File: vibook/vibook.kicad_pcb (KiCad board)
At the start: 2 copper layers, 15 x 89.5 mm, 53 parts, among them IC3 STLQ020C33R, J1 Conn_ARM_JTAG_SWD_10, SW3 SW_Push, U2 STM32L011K4Ux, U3 MPR121QR2, U5 MPR121QR2

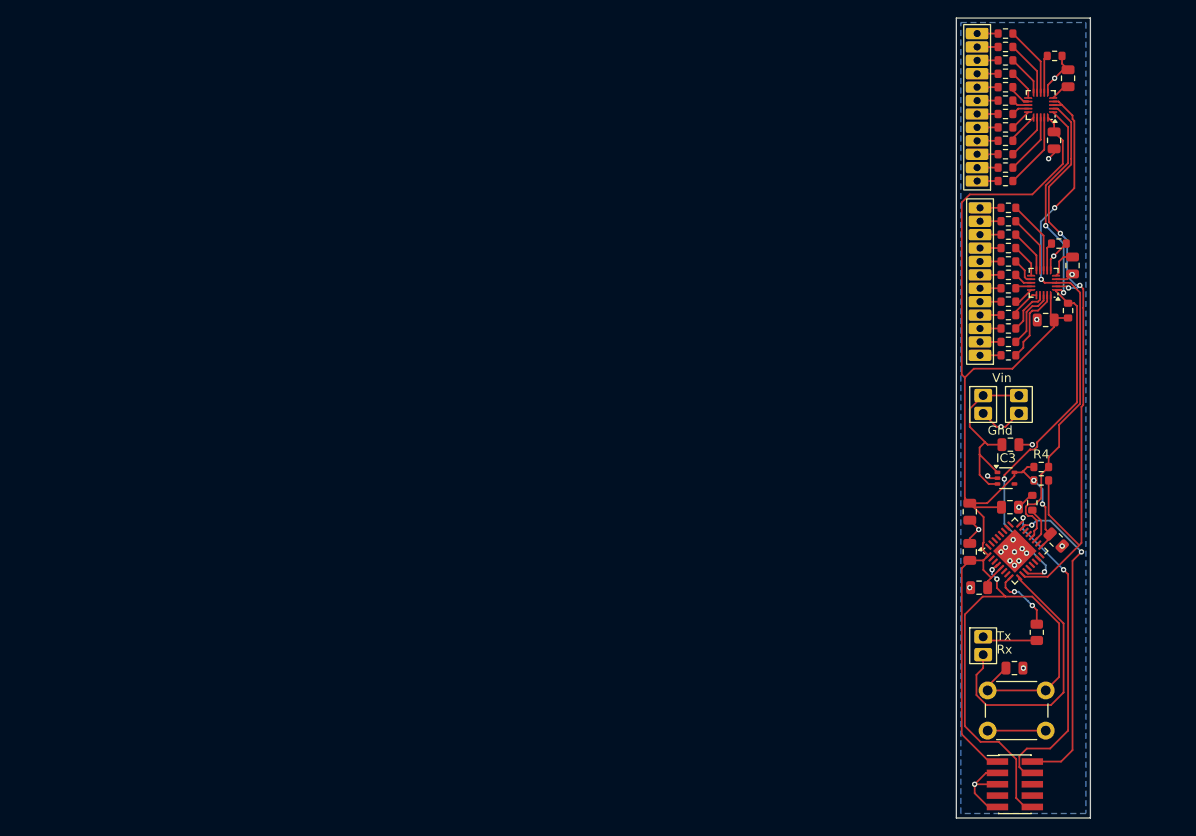
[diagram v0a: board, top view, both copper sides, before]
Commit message: updated board design
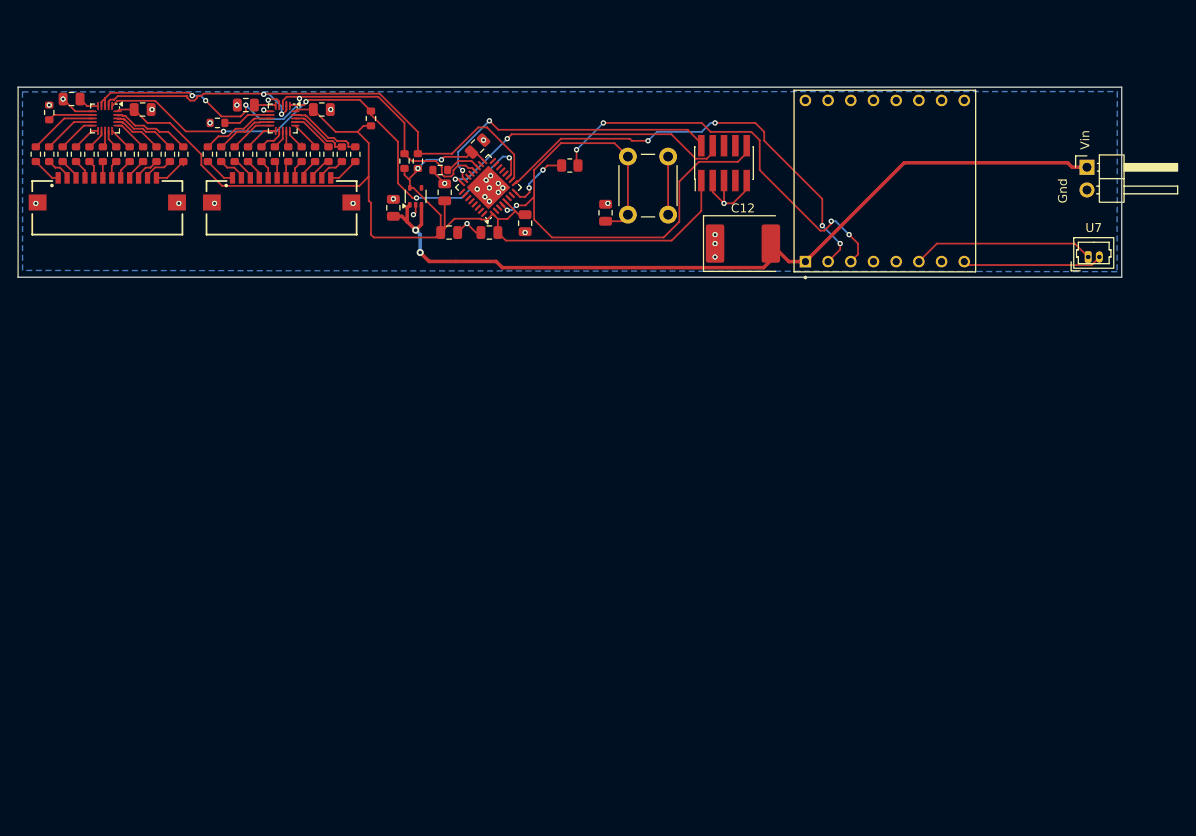
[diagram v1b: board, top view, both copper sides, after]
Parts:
- removed U1, U4: ~, jlc:12matrix
- added C12: 470u, Capacitor_Tantalum_SMD:CP_EIA-7360-38_Kemet-E, F.Cu at (102.6, 111.5)
- added J2: 6861XX148922_686112148922, 6861XX148922_686112148922:686112148922, F.Cu at (51.0, 107.5)
- added J3: 6861XX148922_686112148922, 6861XX148922_686112148922:686112148922, F.Cu at (31.5, 107.5)
- U6: value ~ -> DFR0299; footprint jlc:2pin -> DFR0299:MODULE_DFR0299
- U7: footprint jlc:2pin -> Connector_Molex:Molex_PicoBlade_53047-0210_1x02_P1.25mm_Vertical
- U9: footprint jlc:2pin -> Connector_PinHeader_2.54mm:PinHeader_1x02_P2.54mm_Horizontal
- moved R2 112.7 mm to (25.0, 96.8), turned to -90 degrees
- moved C11 111.5 mm to (27.5, 95.3), turned to 180 degrees
- moved R19 109.3 mm to (23.5, 101.5), turned to -90 degrees
- moved R20 107.7 mm to (25.0, 101.5), turned to -90 degrees
- moved R21 106.0 mm to (26.5, 101.5), turned to -90 degrees
- moved U5 104.7 mm to (31.2, 97.5), turned to -90 degrees
- moved R22 104.4 mm to (28.0, 101.5), turned to -90 degrees
- moved R23 102.8 mm to (29.5, 101.5), turned to -90 degrees
- moved C7 102.0 mm to (35.5, 96.5), turned to 180 degrees
- moved R24 101.2 mm to (31.0, 101.5), turned to -90 degrees
- moved R25 99.6 mm to (32.5, 101.5), turned to -90 degrees
- moved R26 98.0 mm to (34.0, 101.5), turned to -90 degrees
- moved R27 96.5 mm to (35.5, 101.5), turned to -90 degrees
- moved R3 95.1 mm to (43.8, 98.0), turned to 0 degrees
- moved R28 95.0 mm to (37.0, 101.5), turned to -90 degrees
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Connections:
- C6 pad 2: Net-(IC3-EN) -> +4.5V
- IC3 pad 1: Net-(IC3-EN) -> +4.5V
- IC3 pad 3: Net-(IC3-EN) -> +4.5V
- R31 pad 1: Net-(U6-P1) -> Net-(U6-TX)
- U6 pad 1: Net-(U6-P1) -> +4.5V
- U7 pad 1: Net-(IC3-EN) -> Net-(U6-SPK1)
- U7 pad 2: GND -> Net-(U6-SPK2)
- U9 pad 1: Net-(IC3-EN) -> +4.5V
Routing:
- net +4.5V: track 0.00 -> 93.5 mm, vias 0 -> 2
- net Net-(U6-TX): track 0.00 -> 45.2 mm, vias 0 -> 4
- net Net-(IC3-EN): track 21.7 -> 0.00 mm
- net Net-(U6-SPK1): track 0.00 -> 20.4 mm
- net Net-(U2-PA3): track 30.5 -> 49.9 mm, vias 0 -> 4
- net Net-(U6-SPK2): track 0.00 -> 15.7 mm
- net GND: track 44.8 -> 33.3 mm, vias 23 -> 32
- net Net-(U2-PA4): track 72.5 -> 61.7 mm, vias 3 -> 2
- net Net-(U6-P1): track 6.17 -> 0.00 mm
- net +3.3V: track 133.2 -> 128.4 mm
- net Net-(J1-SWDIO/TMS): track 36.0 -> 32.8 mm
- net Net-(U2-PA5): track 64.8 -> 61.8 mm
- net Net-(U2-PA10): track 60.2 -> 57.3 mm, vias 2 -> 4
- net Net-(J1-~{RESET}): track 63.1 -> 65.8 mm
- net Net-(U3-REXT): track 3.20 -> 5.64 mm
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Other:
- board size 15 x 89.5 mm -> 123.5 x 21.3 mm
- board text removed: "Rx"
- board text removed: "Tx"
